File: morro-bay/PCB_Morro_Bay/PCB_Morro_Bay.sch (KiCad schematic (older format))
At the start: 40 parts, among them J1 USB_B, J2 Conn_01x02, U1 MCP2515-xSO, U2 SN65HVD232, U3 MIC5504-3.3YM5, U4 ATSAMD21J18A-AU, Y1 Crystal, Y2 Crystal, Y3 Crystal

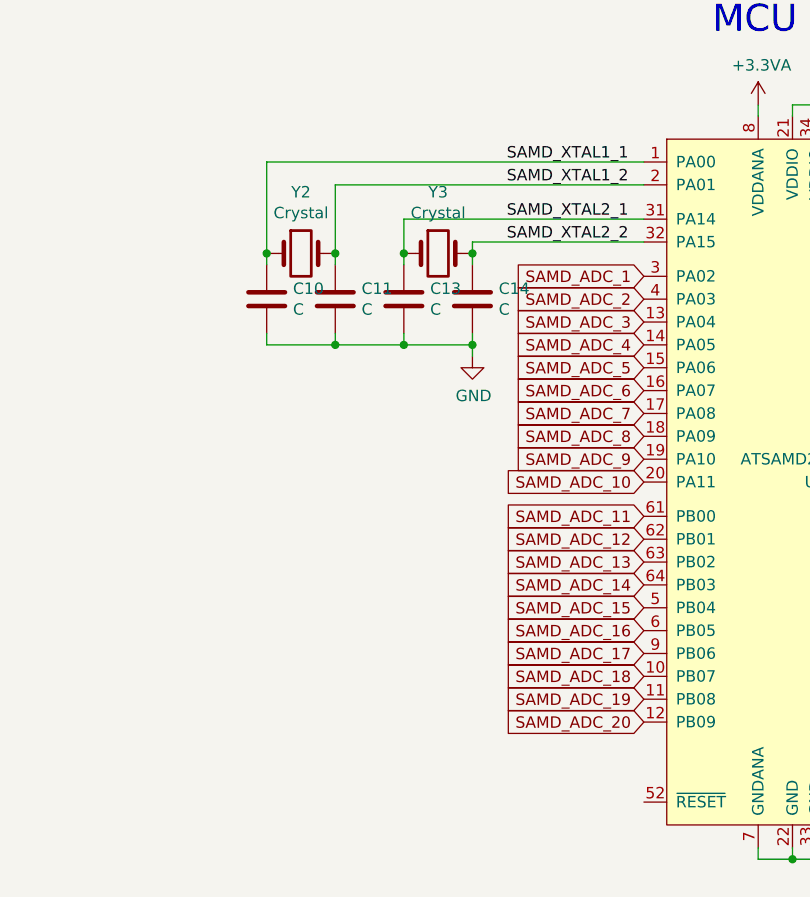
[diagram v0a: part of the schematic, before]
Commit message: Work on analog inputs
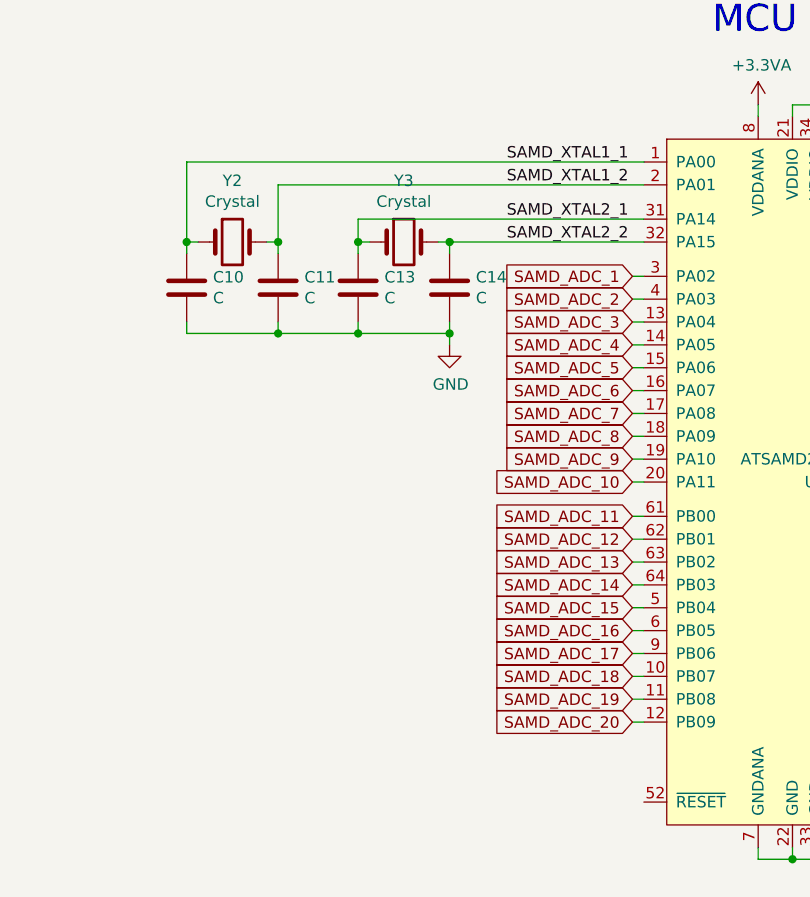
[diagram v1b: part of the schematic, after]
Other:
- moved on the sheet: C10, C11, C13, C14, Y2, Y3
